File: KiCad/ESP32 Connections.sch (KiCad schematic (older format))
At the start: 6 parts

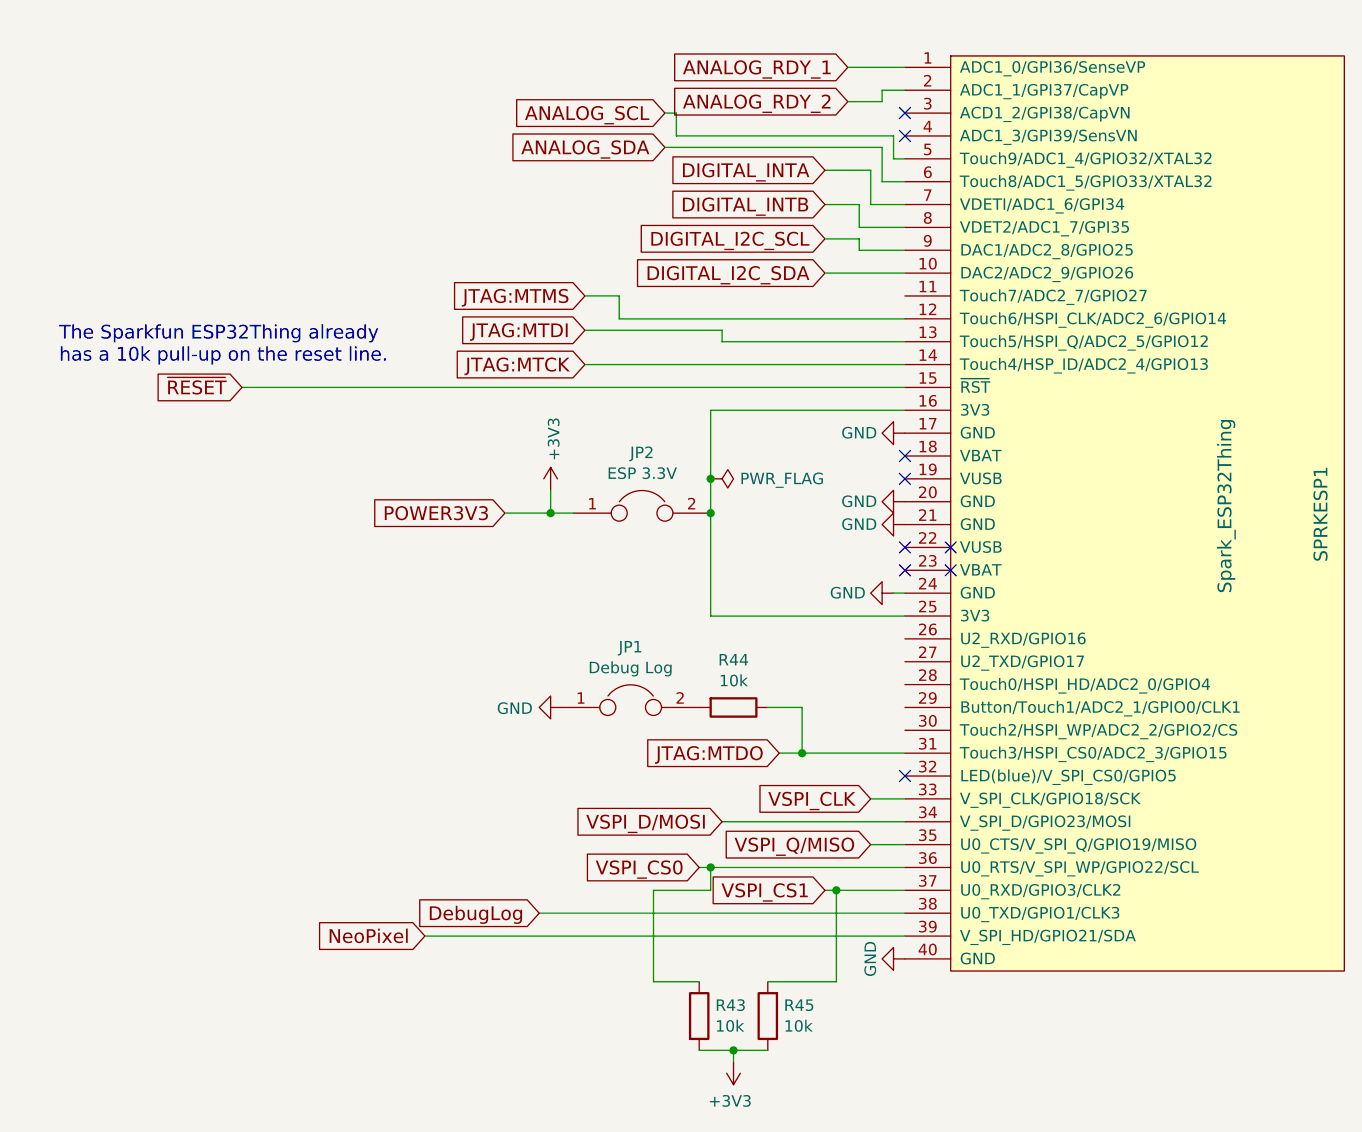
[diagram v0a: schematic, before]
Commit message: More work
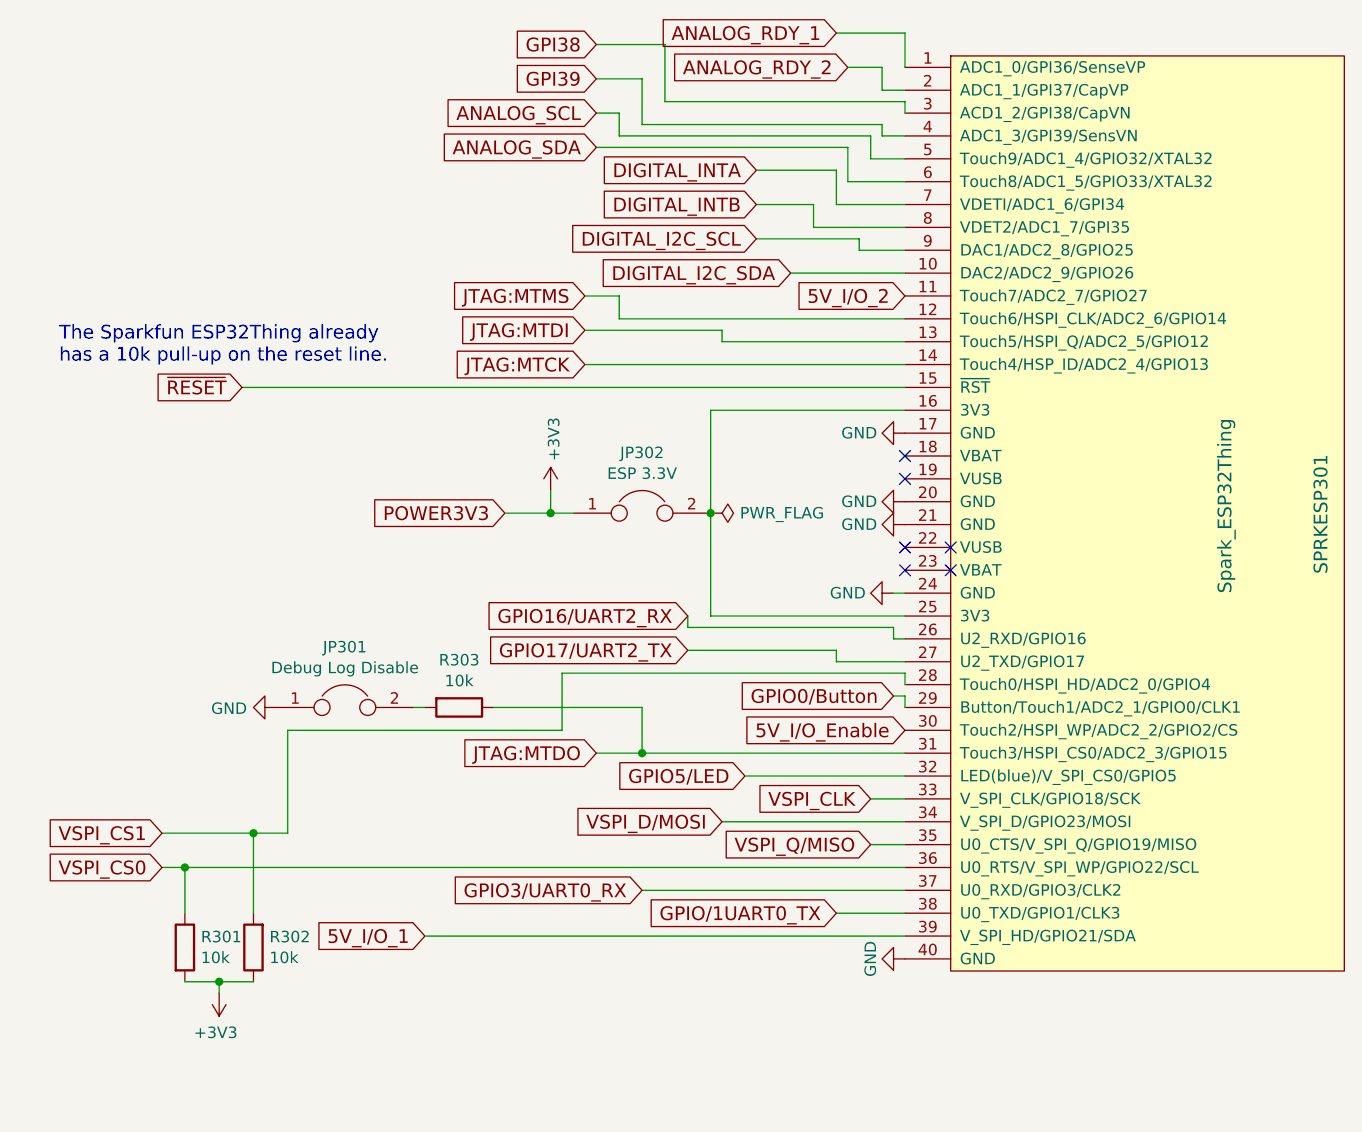
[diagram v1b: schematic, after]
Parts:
- JP301: renamed from JP1; value Debug Log -> Debug Log Disable
- renumbered JP2 to JP302, R43 to R301, R45 to R302, R44 to R303, SPRKESP1 to SPRKESP301
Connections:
- net VSPI_CS1: now also SPRKESP301.28 (Touch0/HSPI_HD/ADC2_0/GPIO4); no longer SPRKESP301.37 (U0_RXD/GPIO3/CLK2)
- net 5V_I/O_2: now reaches SPRKESP301.11 (Touch7/ADC2_7/GPIO27)
- net GPIO16/UART2_RX: now reaches SPRKESP301.26 (U2_RXD/GPIO16)
- net GPIO17/UART2_TX: now reaches SPRKESP301.27 (U2_TXD/GPIO17)
- net GPIO0/Button: now reaches SPRKESP301.29 (Button/Touch1/ADC2_1/GPIO0/CLK1)
- net GPI38: now reaches SPRKESP301.3 (ACD1_2/GPI38/CapVN)
- net 5V_I/O_Enable: now reaches SPRKESP301.30 (Touch2/HSPI_WP/ADC2_2/GPIO2/CS)
- net GPIO5/LED: now reaches SPRKESP301.32 (LED(blue)/V_SPI_CS0/GPIO5)
- net GPI39: now reaches SPRKESP301.4 (ADC1_3/GPI39/SensVN)
- net DebugLog renamed GPIO/1UART0_TX
- net NeoPixel renamed 5V_I/O_1
- new net GPIO3/UART0_RX: SPRKESP301.37 (U0_RXD/GPIO3/CLK2)
- no-connect marks 9 -> 6
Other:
- moved on the sheet: JP301, R301, R302, R303
